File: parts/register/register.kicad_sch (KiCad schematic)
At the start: 33 parts

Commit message: Update High Level
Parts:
- C1, C11, C2: footprint (none) -> Capacitor_SMD:C_0805_2012Metric
- D10, D11, D12, D13, D14, D15, D16, D17: footprint (none) -> LED_THT:LED_D5.0mm
- H1, H2, H3, H4: footprint (none) -> MountingHole:MountingHole_2.2mm_M2_DIN965_Pad
- J1, J6: footprint (none) -> Connector_PinHeader_2.54mm:PinHeader_1x08_P2.54mm_Vertical
- J2, J3, J4, J5: footprint (none) -> Connector_PinHeader_2.54mm:PinHeader_1x01_P2.54mm_Vertical
- J7: footprint (none) -> Connector_PinHeader_2.54mm:PinHeader_1x02_P2.54mm_Vertical
- R24, R25, R26, R27, R28, R29, R30, R31: footprint (none) -> Resistor_SMD:R_0805_2012Metric
- U1: footprint (none) -> Package_DIP:DIP-20_W7.62mm
- U2, U3: footprint (none) -> Package_DIP:DIP-16_W7.62mm
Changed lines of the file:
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@@
     (property "Reference" "D12" (id 0) (at 111.76 142.24 0))
     (property "Value" "~" (id 1) (at 116.84 142.24 0))
-    (property "Footprint" "" (id 2) (at 114.3 142.24 0)
+    (property "Footprint" "LED_THT:LED_D5.0mm" (id 2) (at 114.3 142.24 0)
       (effects (font (size 1.27 1.27)) hide)
     )
@@
     (property "Reference" "D16" (id 0) (at 142.24 142.24 0))
     (property "Value" "~" (id 1) (at 147.32 142.24 0))
-    (property "Footprint" "" (id 2) (at 144.78 142.24 0)
+    (property "Footprint" "LED_THT:LED_D5.0mm" (id 2) (at 144.78 142.24 0)
       (effects (font (size 1.27 1.27)) hide)
     )
@@
     (property "Reference" "D17" (id 0) (at 149.86 142.24 0))
     (property "Value" "~" (id 1) (at 154.94 142.24 0))
-    (property "Footprint" "" (id 2) (at 152.4 142.24 0)
+    (property "Footprint" "LED_THT:LED_D5.0mm" (id 2) (at 152.4 142.24 0)
       (effects (font (size 1.27 1.27)) hide)
     )
@@
     (property "Reference" "R26" (id 0) (at 116.332 153.67 90))
     (property "Value" "~" (id 1) (at 114.3 153.67 90))
-    (property "Footprint" "" (id 2) (at 112.522 153.67 90)
+    (property "Footprint" "Resistor_SMD:R_0805_2012Metric" (id 2) (at 112.522 153.67 90)
       (effects (font (size 1.27 1.27)) hide)
     )
@@
     (property "Reference" "R27" (id 0) (at 123.952 153.67 90))
     (property "Value" "~" (id 1) (at 121.92 153.67 90))
-    (property "Footprint" "" (id 2) (at 120.142 153.67 90)
+    (property "Footprint" "Resistor_SMD:R_0805_2012Metric" (id 2) (at 120.142 153.67 90)
       (effects (font (size 1.27 1.27)) hide)
     )
@@
     (property "Reference" "R29" (id 0) (at 139.192 153.67 90))
     (property "Value" "~" (id 1) (at 137.16 153.67 90))
-    (property "Footprint" "" (id 2) (at 135.382 153.67 90)
+    (property "Footprint" "Resistor_SMD:R_0805_2012Metric" (id 2) (at 135.382 153.67 90)
       (effects (font (size 1.27 1.27)) hide)
     )
@@
     (property "Reference" "R31" (id 0) (at 154.432 153.67 90))
     (property "Value" "~" (id 1) (at 152.4 153.67 90))
-    (property "Footprint" "" (id 2) (at 150.622 153.67 90)
+    (property "Footprint" "Resistor_SMD:R_0805_2012Metric" (id 2) (at 150.622 153.67 90)
       (effects (font (size 1.27 1.27)) hide)
     )
@@
     (property "Reference" "D10" (id 0) (at 96.52 142.24 0))
     (property "Value" "~" (id 1) (at 101.6 142.24 0))
-    (property "Footprint" "" (id 2) (at 99.06 142.24 0)
+    (property "Footprint" "LED_THT:LED_D5.0mm" (id 2) (at 99.06 142.24 0)
       (effects (font (size 1.27 1.27)) hide)
     )
@@
     (property "Reference" "D11" (id 0) (at 104.14 142.24 0))
     (property "Value" "~" (id 1) (at 109.22 142.24 0))
-    (property "Footprint" "" (id 2) (at 106.68 142.24 0)
+    (property "Footprint" "LED_THT:LED_D5.0mm" (id 2) (at 106.68 142.24 0)
       (effects (font (size 1.27 1.27)) hide)
     )
@@
     (property "Reference" "D13" (id 0) (at 119.38 142.24 0))
     (property "Value" "~" (id 1) (at 124.46 142.24 0))
-    (property "Footprint" "" (id 2) (at 121.92 142.24 0)
+    (property "Footprint" "LED_THT:LED_D5.0mm" (id 2) (at 121.92 142.24 0)
       (effects (font (size 1.27 1.27)) hide)
     )
@@
     (property "Reference" "D14" (id 0) (at 127 142.24 0))
     (property "Value" "~" (id 1) (at 132.08 142.24 0))
-    (property "Footprint" "" (id 2) (at 129.54 142.24 0)
+    (property "Footprint" "LED_THT:LED_D5.0mm" (id 2) (at 129.54 142.24 0)
       (effects (font (size 1.27 1.27)) hide)
     )
@@
     (property "Reference" "D15" (id 0) (at 134.62 142.24 0))
     (property "Value" "~" (id 1) (at 139.7 142.24 0))
-    (property "Footprint" "" (id 2) (at 137.16 142.24 0)
+    (property "Footprint" "LED_THT:LED_D5.0mm" (id 2) (at 137.16 142.24 0)
       (effects (font (size 1.27 1.27)) hide)
     )
@@
     (property "Reference" "R24" (id 0) (at 101.092 153.67 90))
     (property "Value" "~" (id 1) (at 99.06 153.67 90))
-    (property "Footprint" "" (id 2) (at 97.282 153.67 90)
+    (property "Footprint" "Resistor_SMD:R_0805_2012Metric" (id 2) (at 97.282 153.67 90)
       (effects (font (size 1.27 1.27)) hide)
     )
@@
     (property "Reference" "R25" (id 0) (at 108.712 153.67 90))
     (property "Value" "~" (id 1) (at 106.68 153.67 90))
-    (property "Footprint" "" (id 2) (at 104.902 153.67 90)
+    (property "Footprint" "Resistor_SMD:R_0805_2012Metric" (id 2) (at 104.902 153.67 90)
       (effects (font (size 1.27 1.27)) hide)
     )
@@
     (property "Reference" "R28" (id 0) (at 131.572 153.67 90))
     (property "Value" "~" (id 1) (at 129.54 153.67 90))
-    (property "Footprint" "" (id 2) (at 127.762 153.67 90)
+    (property "Footprint" "Resistor_SMD:R_0805_2012Metric" (id 2) (at 127.762 153.67 90)
       (effects (font (size 1.27 1.27)) hide)
     )
@@
     (property "Reference" "R30" (id 0) (at 146.812 153.67 90))
     (property "Value" "~" (id 1) (at 144.78 153.67 90))
-    (property "Footprint" "" (id 2) (at 143.002 153.67 90)
+    (property "Footprint" "Resistor_SMD:R_0805_2012Metric" (id 2) (at 143.002 153.67 90)
       (effects (font (size 1.27 1.27)) hide)
     )
@@
       (effects (font (size 1.27 1.27)) (justify left))
     )
-    (property "Footprint" "" (id 2) (at 232.1052 71.12 0)
+    (property "Footprint" "Capacitor_SMD:C_0805_2012Metric" (id 2) (at 232.1052 71.12 0)
       (effects (font (size 1.27 1.27)) hide)
     )
@@
       (effects (font (size 1.27 1.27)) (justify right))
     )
-    (property "Footprint" "" (id 2) (at 91.44 67.31 0)
+    (property "Footprint" "Package_DIP:DIP-20_W7.62mm" (id 2) (at 91.44 67.31 0)
       (effects (font (size 1.27 1.27)) hide)
     )
@@
     (property "Reference" "J7" (id 0) (at 221.7928 60.325 0))
     (property "Value" "~" (id 1) (at 221.7928 62.6364 0))
-    (property "Footprint" "" (id 2) (at 219.71 68.58 0)
+    (property "Footprint" "Connector_PinHeader_2.54mm:PinHeader_1x02_P2.54mm_Vertical" (id 2) (at 219.71 68.58 0)
       (effects (font (size 1.27 1.27)) hide)
     )
@@
       (effects (font (size 1.27 1.27)) (justify left))
     )
-    (property "Footprint" "" (id 2) (at 134.62 67.31 0)
+    (property "Footprint" "Package_DIP:DIP-16_W7.62mm" (id 2) (at 134.62 67.31 0)
       (effects (font (size 1.27 1.27)) hide)
     )
@@
       (effects (font (size 1.27 1.27)) (justify left))
     )
-    (property "Footprint" "" (id 2) (at 186.69 67.31 0)
+    (property "Footprint" "Package_DIP:DIP-16_W7.62mm" (id 2) (at 186.69 67.31 0)
       (effects (font (size 1.27 1.27)) hide)
     )
@@
       (effects (font (size 1.27 1.27)) (justify left))
     )
-    (property "Footprint" "" (id 2) (at 254 76.2 0)
+    (property "Footprint" "MountingHole:MountingHole_2.2mm_M2_DIN965_Pad" (id 2) (at 254 76.2 0)
       (effects (font (size 1.27 1.27)) hide)
     )
@@
       (effects (font (size 1.27 1.27)) (justify left))
     )
-    (property "Footprint" "" (id 2) (at 248.92 76.2 0)
+    (property "Footprint" "MountingHole:MountingHole_2.2mm_M2_DIN965_Pad" (id 2) (at 248.92 76.2 0)
       (effects (font (size 1.27 1.27)) hide)
     )
@@
       (effects (font (size 1.27 1.27)) (justify left))
     )
-    (property "Footprint" "" (id 2) (at 243.84 76.2 0)
+    (property "Footprint" "MountingHole:MountingHole_2.2mm_M2_DIN965_Pad" (id 2) (at 243.84 76.2 0)
       (effects (font (size 1.27 1.27)) hide)
     )
@@
       (effects (font (size 1.27 1.27)) (justify left))
     )
-    (property "Footprint" "" (id 2) (at 238.76 76.2 0)
+    (property "Footprint" "MountingHole:MountingHole_2.2mm_M2_DIN965_Pad" (id 2) (at 238.76 76.2 0)
       (effects (font (size 1.27 1.27)) hide)
     )
@@
       (effects (font (size 1.27 1.27)) (justify left))
     )
-    (property "Footprint" "" (id 2) (at 238.4552 71.12 0)
+    (property "Footprint" "Capacitor_SMD:C_0805_2012Metric" (id 2) (at 238.4552 71.12 0)
       (effects (font (size 1.27 1.27)) hide)
     )
@@
       (effects (font (size 1.27 1.27)) (justify left))
     )
-    (property "Footprint" "" (id 2) (at 244.8052 71.12 0)
+    (property "Footprint" "Capacitor_SMD:C_0805_2012Metric" (id 2) (at 244.8052 71.12 0)
       (effects (font (size 1.27 1.27)) hide)
     )
@@
     )
     (property "Value" "~" (id 1) (at 231.14 26.67 0))
-    (property "Footprint" "" (id 2) (at 227.33 25.4 0)
+    (property "Footprint" "Connector_PinHeader_2.54mm:PinHeader_1x08_P2.54mm_Vertical" (id 2) (at 227.33 25.4 0)
       (effects (font (size 1.27 1.27)) hide)
     )
@@
       (effects (font (size 1.27 1.27)) (justify left))
     )
-    (property "Footprint" "" (id 2) (at 170.18 125.73 0)
+    (property "Footprint" "Connector_PinHeader_2.54mm:PinHeader_1x08_P2.54mm_Vertical" (id 2) (at 170.18 125.73 0)
       (effects (font (size 1.27 1.27)) hide)
     )
@@
     )
     (property "Value" "~" (id 1) (at 231.14 40.64 0))
-    (property "Footprint" "" (id 2) (at 227.33 40.64 0)
+    (property "Footprint" "Connector_PinHeader_2.54mm:PinHeader_1x01_P2.54mm_Vertical" (id 2) (at 227.33 40.64 0)
       (effects (font (size 1.27 1.27)) hide)
     )
@@
     )
     (property "Value" "~" (id 1) (at 238.76 38.1 0))
-    (property "Footprint" "" (id 2) (at 234.95 38.1 0)
+    (property "Footprint" "Connector_PinHeader_2.54mm:PinHeader_1x01_P2.54mm_Vertical" (id 2) (at 234.95 38.1 0)
       (effects (font (size 1.27 1.27)) hide)
     )
@@
     )
     (property "Value" "~" (id 1) (at 231.14 45.72 0))
-    (property "Footprint" "" (id 2) (at 227.33 45.72 0)
+    (property "Footprint" "Connector_PinHeader_2.54mm:PinHeader_1x01_P2.54mm_Vertical" (id 2) (at 227.33 45.72 0)
       (effects (font (size 1.27 1.27)) hide)
     )
@@
     )
     (property "Value" "~" (id 1) (at 217.17 93.98 0))
-    (property "Footprint" "" (id 2) (at 213.36 93.98 0)
-      (effects (font (size 1.27 1.27)) hide)
-    )
+    (property "Footprint" "Connector_PinHeader_2.54mm:PinHeader_1x01_P2.54mm_Vertical" (id 2) (at 213.36 93.98 0)
+      (effects (font (size 1.27 1.27)) hide)
+    )

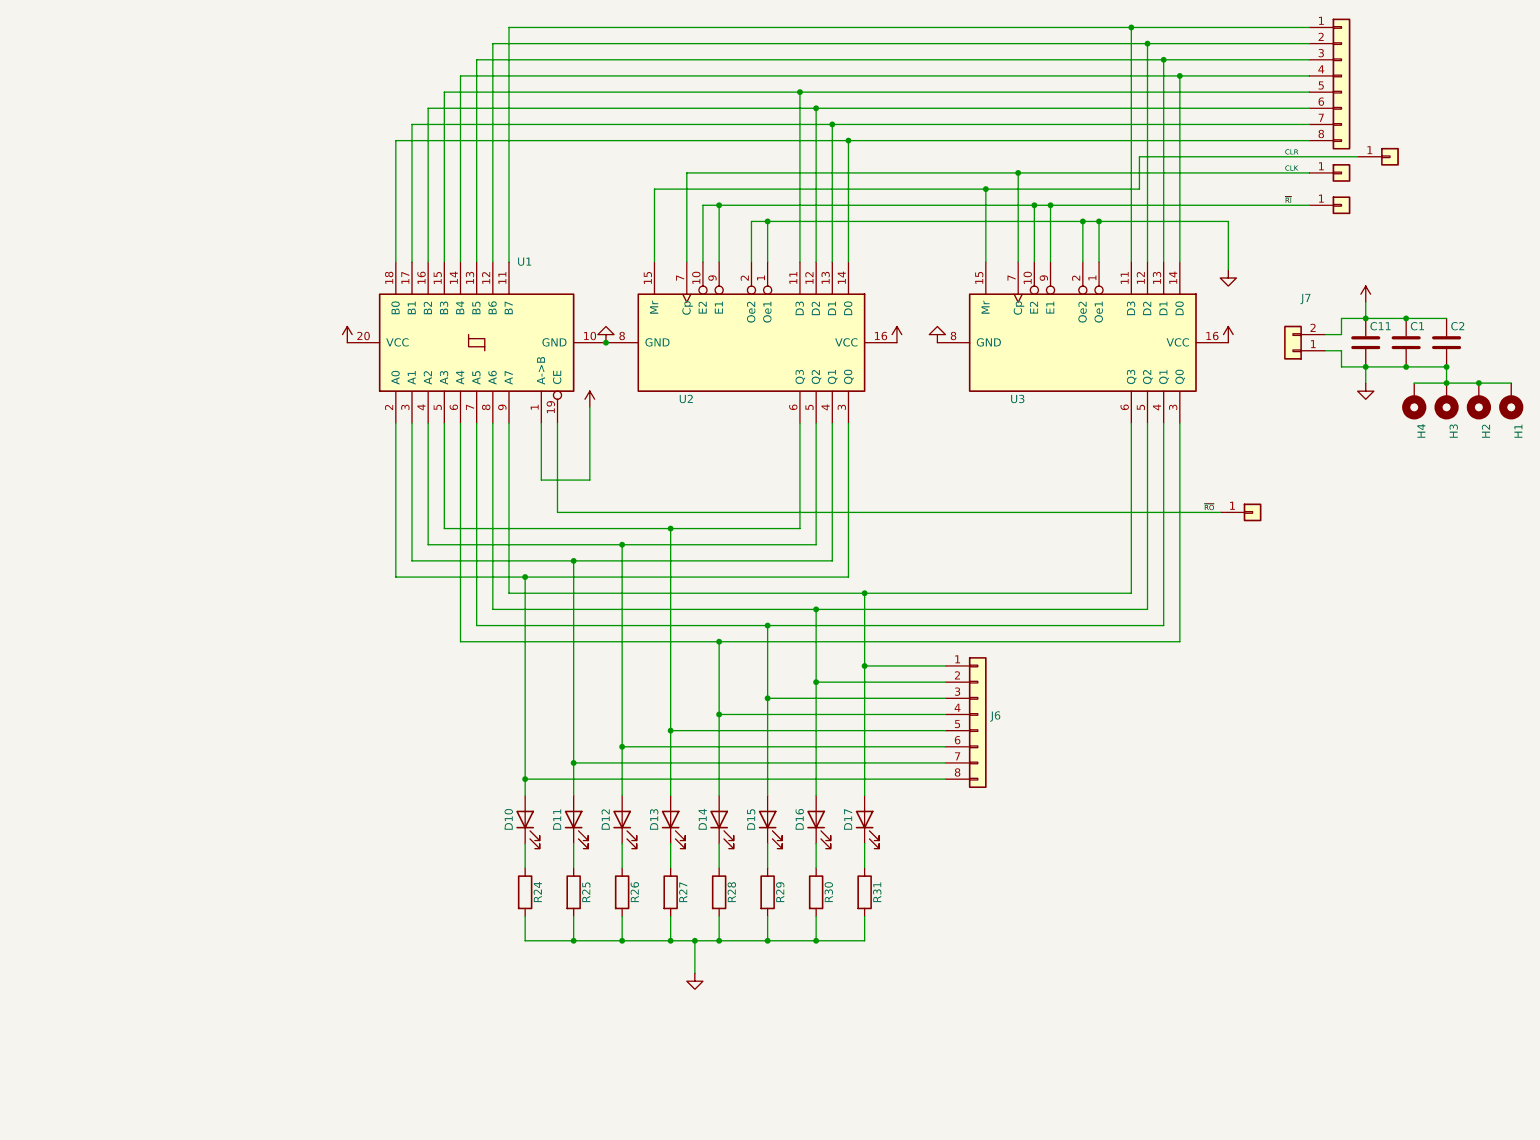
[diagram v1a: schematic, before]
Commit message: SMD Register
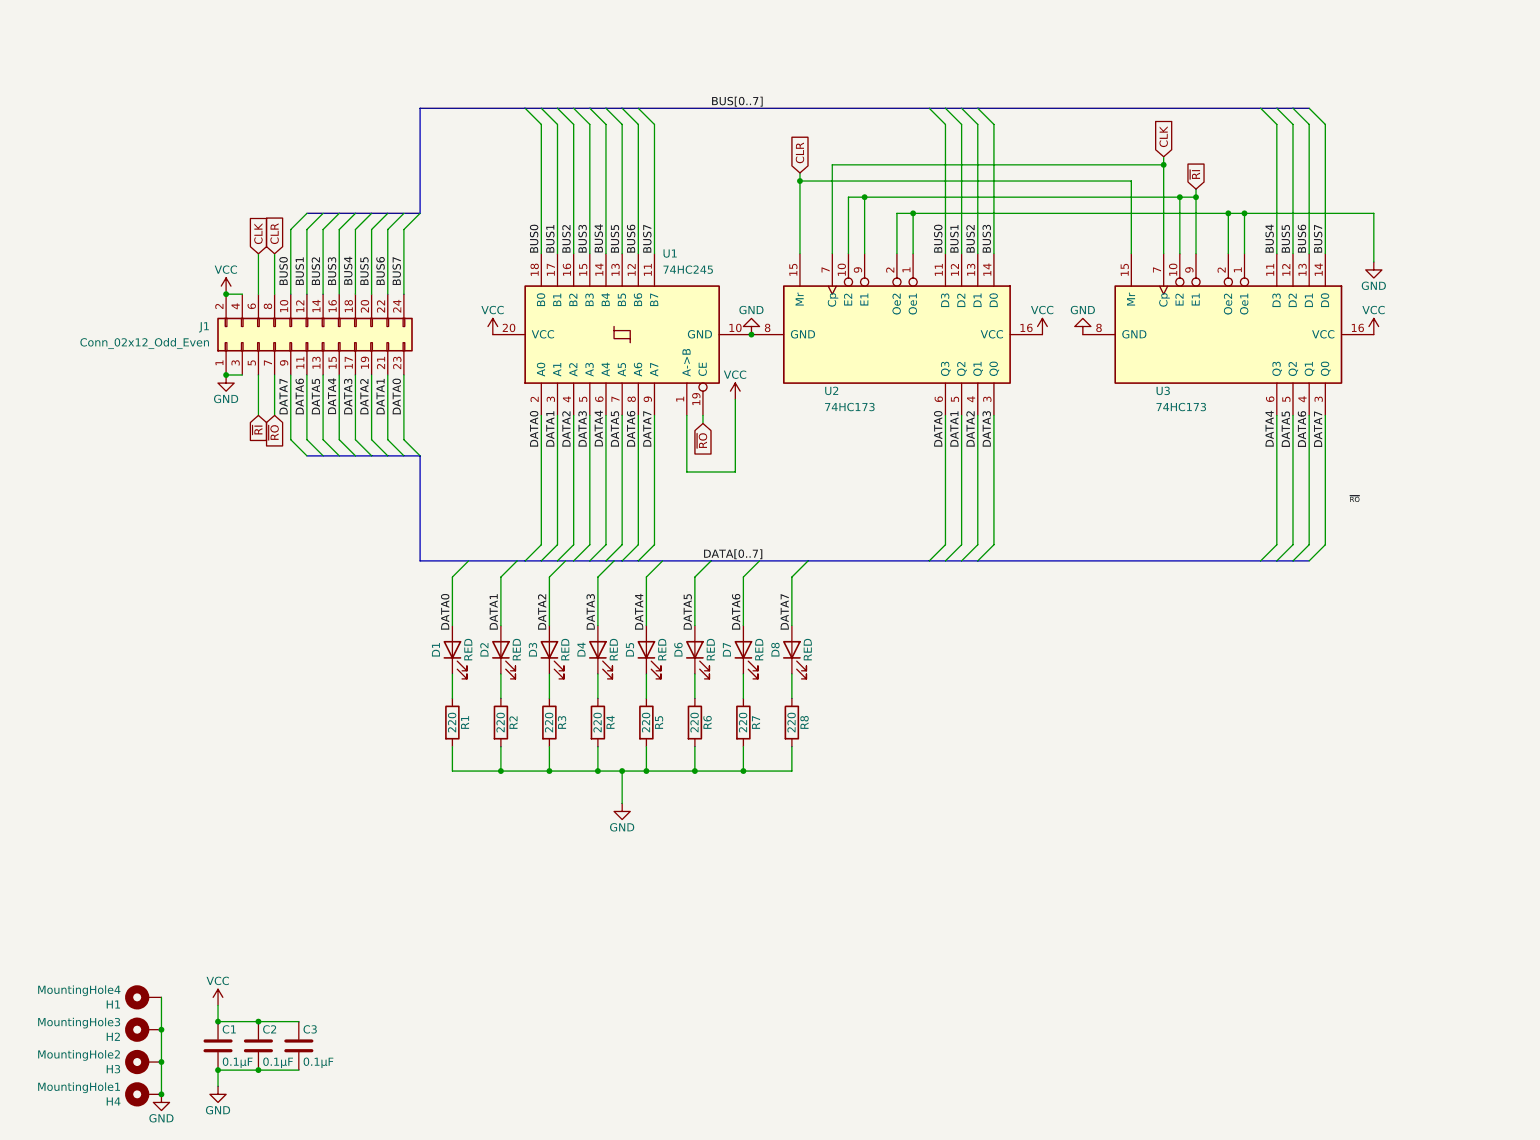
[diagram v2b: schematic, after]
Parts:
- removed D10, D11, D12, D13, D14, D15, D16, D17: ~, LED_THT:LED_D5.0mm, symbol Device:LED
- removed J1, J6: ~, Connector_PinHeader_2.54mm:PinHeader_1x08_P2.54mm_Vertical, symbol Connector_Generic:Conn_01x08
- removed J2, J3, J4, J5: ~, Connector_PinHeader_2.54mm:PinHeader_1x01_P2.54mm_Vertical, symbol Connector_Generic:Conn_01x01
- removed J7: ~, Connector_PinHeader_2.54mm:PinHeader_1x02_P2.54mm_Vertical, symbol Connector_Generic:Conn_01x02
- removed R24, R25, R26, R27, R28, R29, R30, R31: ~, Resistor_SMD:R_0805_2012Metric, symbol Device:R
- added D1, D2, D3, D4, D5, D6, D7, D8: RED, LED_SMD:LED_0805_2012Metric, symbol Device:LED
- added J1: Conn_02x12_Odd_Even, Connector_IDC:IDC-Header_2x12_P2.54mm_Vertical, symbol Connector_Generic:Conn_02x12_Odd_Even
- added R1, R2, R3, R4, R5, R6, R7, R8: 220, Resistor_SMD:R_0805_2012Metric, symbol Device:R
- C1: renamed from C11; value ~ -> 0.1µF
- C2: renamed from C1; value ~ -> 0.1µF
- C3: renamed from C2; value ~ -> 0.1µF
- H1: value ~ -> MountingHole4; footprint MountingHole:MountingHole_2.2mm_M2_DIN965_Pad -> MountingHole:MountingHole_2.2mm_M2_Pad_Via
- H2: value ~ -> MountingHole3; footprint MountingHole:MountingHole_2.2mm_M2_DIN965_Pad -> MountingHole:MountingHole_2.2mm_M2_Pad_Via
- H3: value ~ -> MountingHole2; footprint MountingHole:MountingHole_2.2mm_M2_DIN965_Pad -> MountingHole:MountingHole_2.2mm_M2_Pad_Via
- H4: value ~ -> MountingHole1; footprint MountingHole:MountingHole_2.2mm_M2_DIN965_Pad -> MountingHole:MountingHole_2.2mm_M2_Pad_Via
- U1: value ~ -> 74HC245; footprint Package_DIP:DIP-20_W7.62mm -> Package_SO:TSSOP-20_4.4x6.5mm_P0.65mm
- U2, U3: value ~ -> 74HC173; footprint Package_DIP:DIP-16_W7.62mm -> Package_SO:SOIC-16_3.9x9.9mm_P1.27mm
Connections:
- net CLK: now also J1.6 (Pin_6)
- net CLR: now also J1.8 (Pin_8)
- net GND: now also J1.1 (Pin_1), J1.3 (Pin_3), R1.2, R2.2, R3.2, R4.2, R5.2, R6.2, R7.2, R8.2
- net VCC: now also J1.2 (Pin_2), J1.4 (Pin_4)
- net ~{RI}: now also J1.5 (Pin_5)
- net ~{RO}: now also J1.7 (Pin_7)
- net DATA1: now reaches U2.5 (Q2)
- net DATA1: now also U1.3 (A1), D2.2 (A), J1.21 (Pin_21); no longer U1.4 (A2)
- net DATA5: now reaches U3.5 (Q2)
- net DATA5: now also U1.7 (A5), D6.2 (A), J1.13 (Pin_13); no longer U1.8 (A6)
- net DATA4: now reaches U3.6 (Q3)
- net DATA4: now also U1.6 (A4), D5.2 (A), J1.15 (Pin_15); no longer U1.9 (A7)
- net DATA0: now reaches U1.2 (A0)
- net DATA0: now also U2.6 (Q3), D1.2 (A), J1.23 (Pin_23); no longer U2.3 (Q0)
- net DATA2: now reaches U2.4 (Q1)
- net DATA2: now also U1.4 (A2), D3.2 (A), J1.19 (Pin_19); no longer U1.3 (A1)
- net DATA3: now reaches U1.5 (A3)
- net DATA3: now also U2.3 (Q0), D4.2 (A), J1.17 (Pin_17); no longer U2.6 (Q3)
- net DATA7: now reaches U3.3 (Q0)
- net DATA7: now also U1.9 (A7), D8.2 (A), J1.9 (Pin_9); no longer U1.6 (A4)
- net DATA6: now reaches U3.4 (Q1)
- net DATA6: now also U1.8 (A6), D7.2 (A), J1.11 (Pin_11); no longer U1.7 (A5)
- net BUS4: now reaches U3.11 (D3)
- net BUS4: now also U1.14 (B4), J1.18 (Pin_18); no longer U1.11 (B7)
- net BUS5: now reaches U3.12 (D2)
- net BUS5: now also U1.13 (B5), J1.20 (Pin_20); no longer U1.12 (B6)
- net BUS6: now reaches U3.13 (D1)
- net BUS6: now also U1.12 (B6), J1.22 (Pin_22); no longer U1.13 (B5)
- net BUS7: now reaches U3.14 (D0)
- net BUS7: now also U1.11 (B7), J1.24 (Pin_24); no longer U1.14 (B4)
- net BUS0: now reaches U2.11 (D3)
- net BUS0: now also U1.18 (B0), J1.10 (Pin_10); no longer U1.15 (B3)
- net BUS1: now reaches U2.12 (D2)
- net BUS1: now also U1.17 (B1), J1.12 (Pin_12); no longer U1.16 (B2)
- net BUS2: now reaches U2.13 (D1)
- net BUS2: now also U1.16 (B2), J1.14 (Pin_14); no longer U1.17 (B1)
- net BUS3: now reaches U2.14 (D0)
- net BUS3: now also U1.15 (B3), J1.16 (Pin_16); no longer U1.18 (B0)
- new net: D8.1 (K), R8.1
- new net: D3.1 (K), R3.1
- new net: D7.1 (K), R7.1
- new net: D2.1 (K), R2.1
- new net: D6.1 (K), R6.1
- new net: D1.1 (K), R1.1
- new net: D5.1 (K), R5.1
- new net: D4.1 (K), R4.1
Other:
- moved on the sheet: C1, C2, C3, U1, U2, U3
